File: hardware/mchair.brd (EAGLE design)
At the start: 25.6 x 53.5 mm, 120 parts, among them J1 UX60-MB-5S8, J2 JTAG-MINI, U1 STM32F769NIH6, U2 S25FS256SAGNFI00, U3 LAN8742A, U4 USB3315C, U5 MIC5503-1.8YMT-TR, U6 MT48LC16M16A2F4, U7 MPM3620GQV-P, U8 NCP186AMX330TAG, X1 G83270021, X2 DSC6101JI2A-025.0000, X3 DSC6101JI2A-024.0000

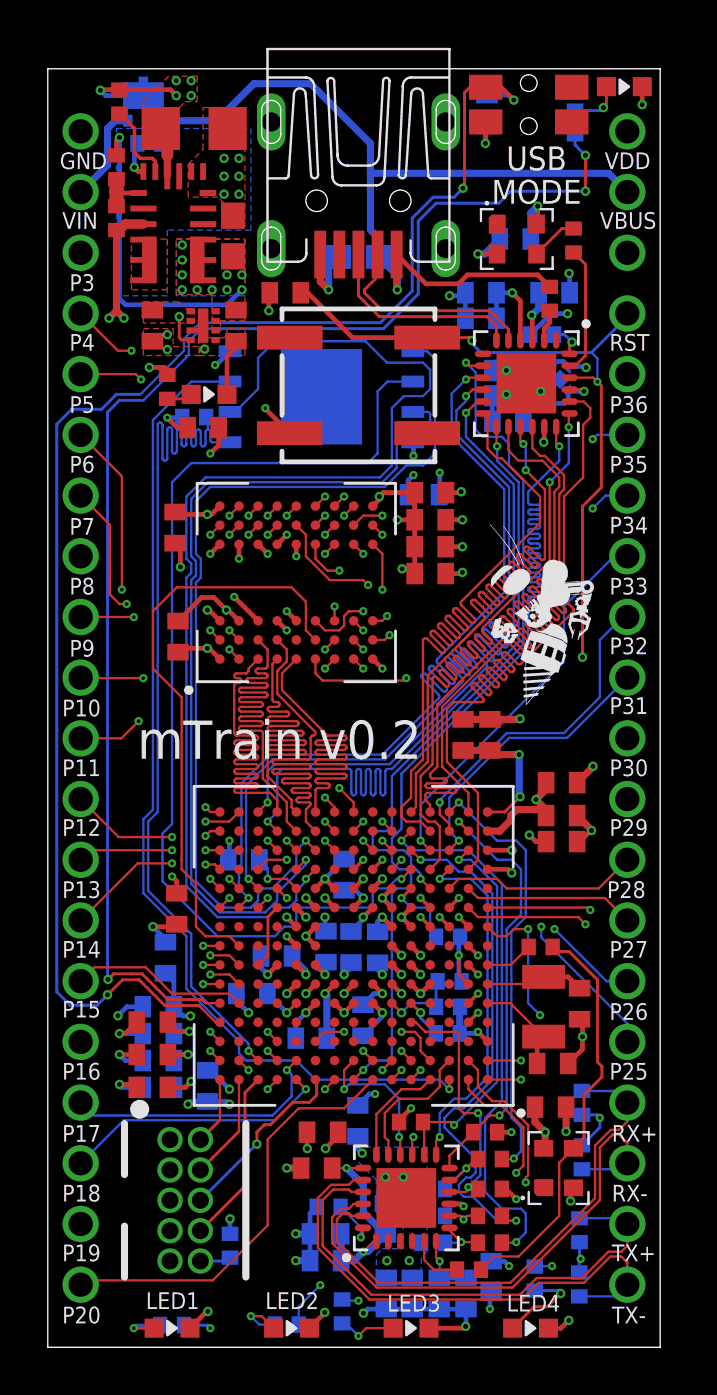
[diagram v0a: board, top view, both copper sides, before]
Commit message: fix drc annular ring
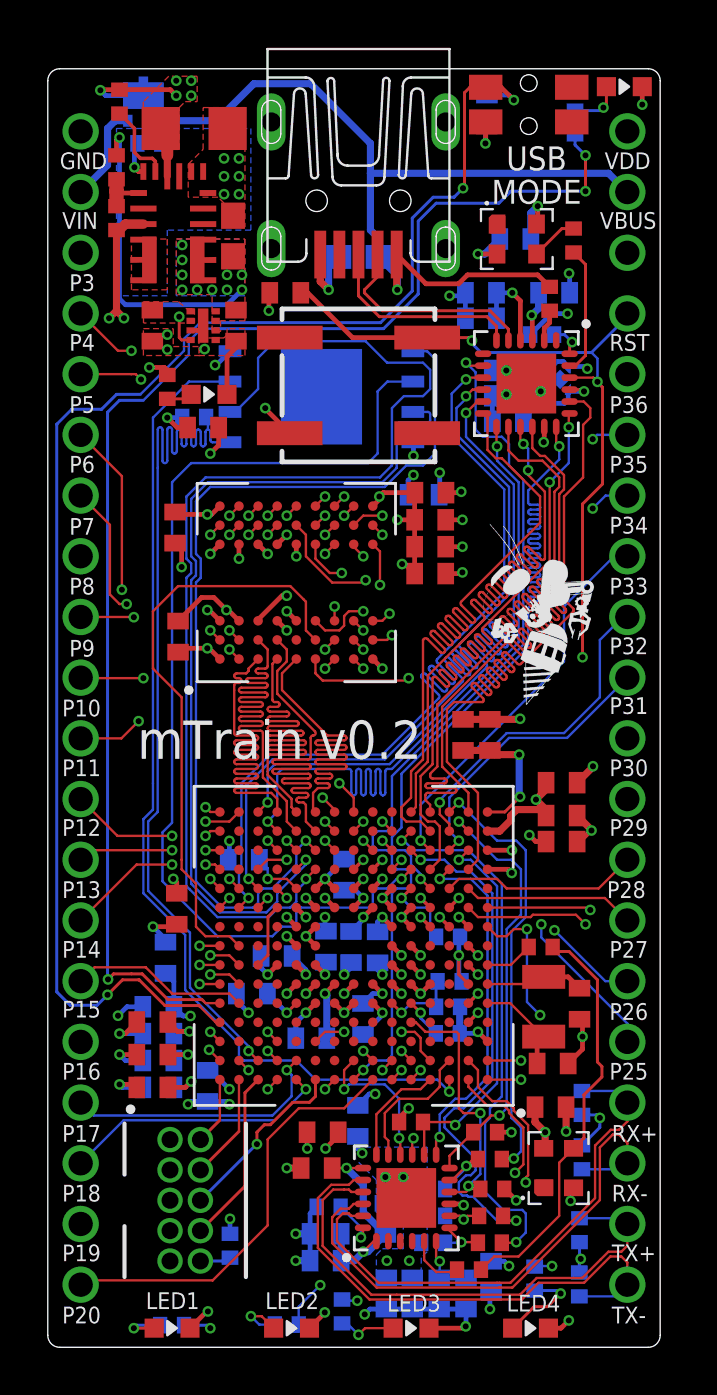
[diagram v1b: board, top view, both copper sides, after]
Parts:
- moved R16 0.10 mm to (18.6, 6.62)
- moved C13 0.05 mm to (13.2, 13.7)
- moved R7 0.05 mm to (18.6, 5.50)
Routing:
- net FMC-A6: track 19.7 -> 18.6 mm
- net FMC-D9: track 19.8 -> 18.7 mm
- net FMC-A5: track 19.9 -> 19.0 mm
- net FMC-SDCKE0: track 20.9 -> 20.2 mm
- net FMC-D13: track 19.2 -> 18.6 mm
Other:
- outline, holes or cut-outs redrawn
